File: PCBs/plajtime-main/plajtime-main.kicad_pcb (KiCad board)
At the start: 6 copper layers, 15.2 x 34 mm, 84 parts, among them J1 RP SWD, J10 Internal connector, J11 USB, J2 RP USB, J4 Display connector, J5 Extention connector, J6 Conn_Coaxial, J7 Battery Connector, J8 Nordic SWD, J9 Conn_Coaxial, U1 W25Q64JWUUIQ, U2 W25Q64JWBYIM, U3 TPS628438YKA, U4 MP2664, U5 RP2350A, U6 BMA456, U7 MAX17055, U9 nRF52833_QDxx, Y1 13MHz, Y2 32MHz, Y3 32.768kHz Crystal

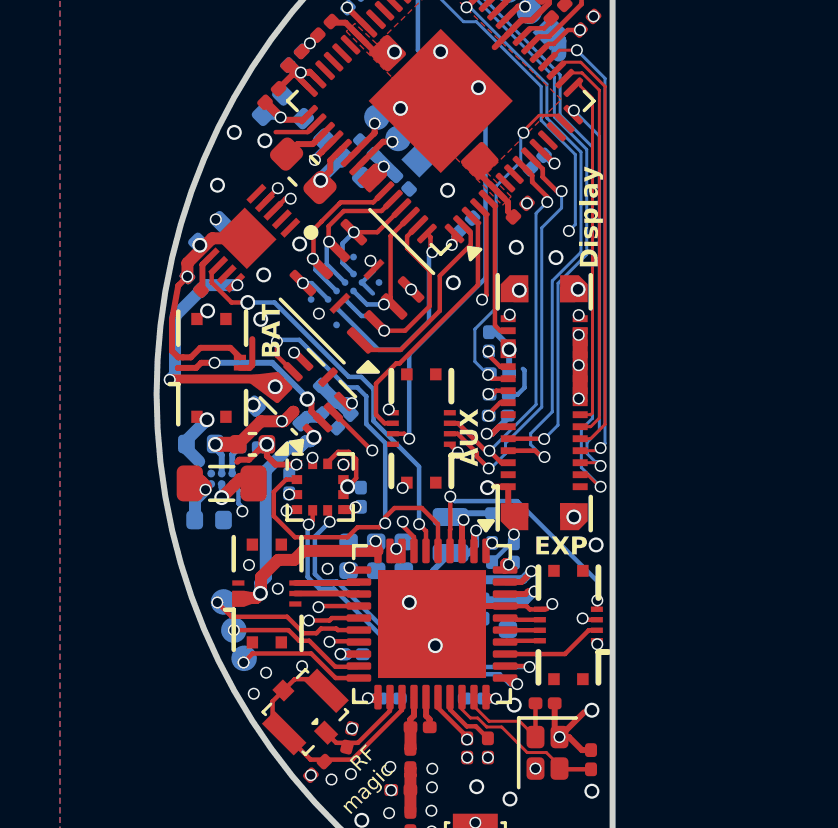
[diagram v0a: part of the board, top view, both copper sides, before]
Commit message: Some fixes after v0.4
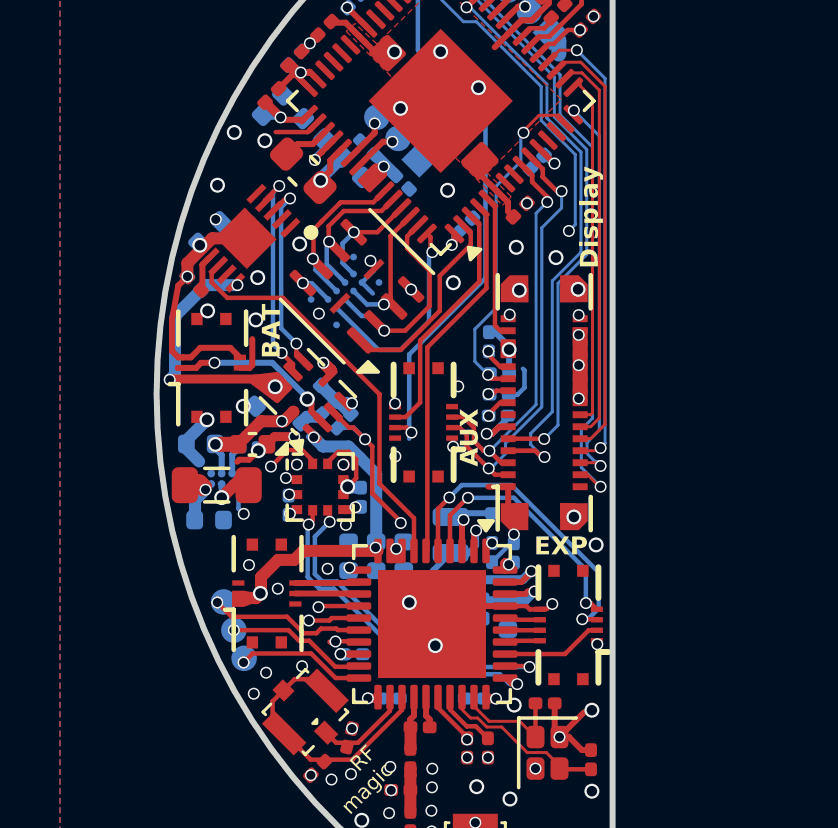
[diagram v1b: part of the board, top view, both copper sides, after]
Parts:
- moved C27 0.72 mm to (-15.8, 3.71), turned to -90 degrees
- moved J10 0.22 mm to (-11.3, 0.94)
- moved L2 0.18 mm to (-18.2, 3.04)
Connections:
- U5 pad 37: /CLK_OUT -> unconnected-(U5-GPIO25-Pad37)
- U9 pad 6: /GAUGE_INT -> GPU_INT
- U9 pad 7: GPU_INT -> /GAUGE_INT
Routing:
- net SCL: track 25.9 -> 32.3 mm
- net /CHARGER_INT: track 9.86 -> 12.2 mm, vias 2 -> 3
- net SDA: track 33.2 -> 31.4 mm, vias 4 -> 5
- net +5V: track 11.9 -> 10.5 mm
- net GPU_INT: track 13.6 -> 12.4 mm, vias 2 -> 0
- net RP_SCL: track 13.8 -> 14.7 mm
- net /SLIDER_INT: track 8.85 -> 8.16 mm
- net RP_SDA: track 13.1 -> 13.7 mm
- net /GAUGE_INT: track 13.6 -> 13.5 mm, vias 2 -> 0
- net GND: track 28.3 -> 28.2 mm, vias 81 -> 84
